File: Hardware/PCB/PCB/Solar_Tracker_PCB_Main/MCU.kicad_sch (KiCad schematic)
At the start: 20 parts, among them IC1 ESP32-S3-WROOM-1-N4R8, IC5 LM1117MPX-3.3_NOPB, J2 USB4940-00-A, J3 1729076, J4 1977223-1, J5 1977223-1

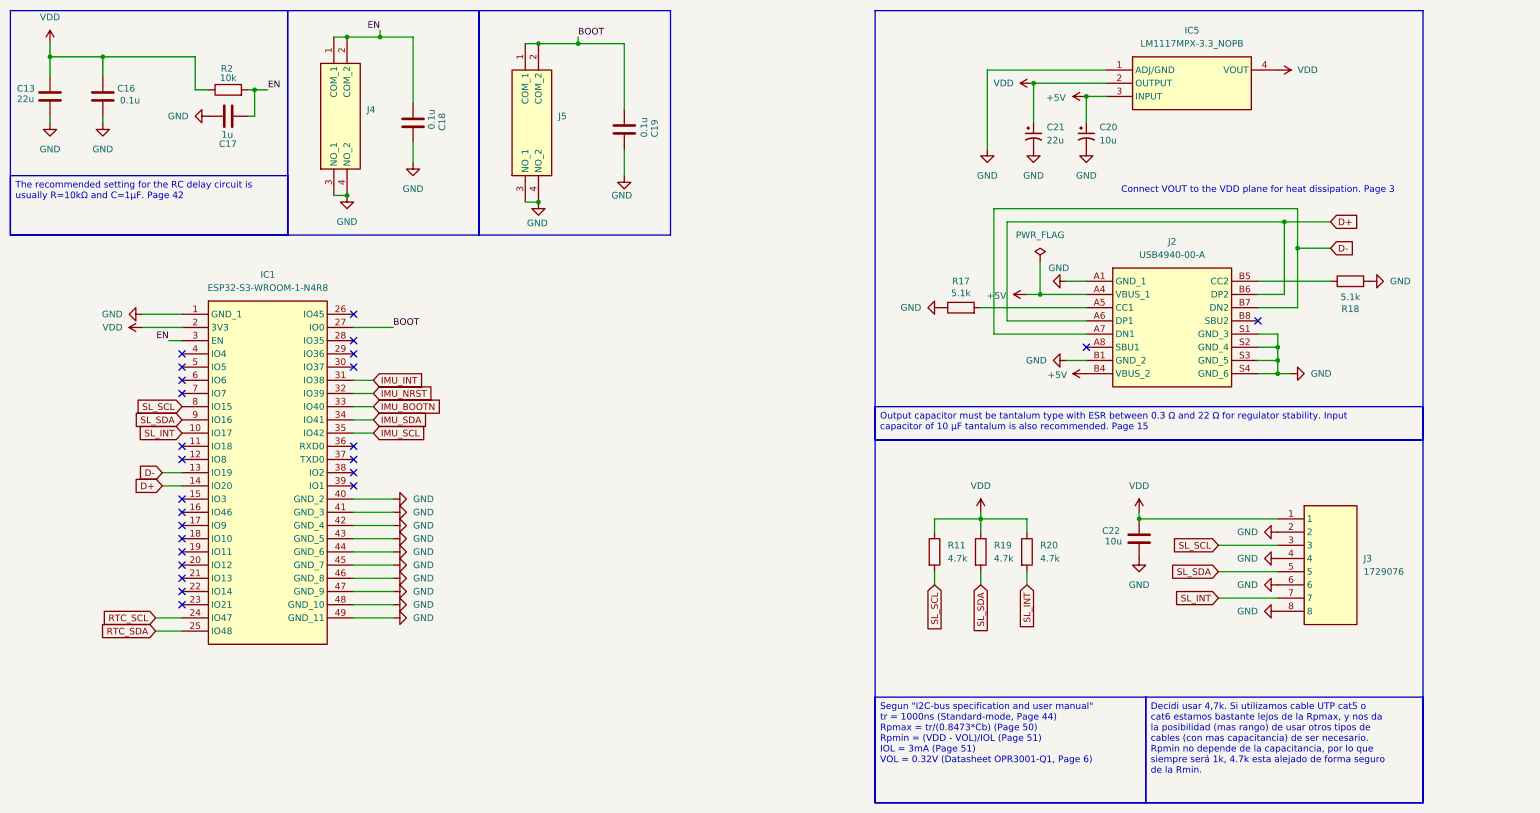
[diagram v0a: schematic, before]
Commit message: comienzo de distribucion pcb
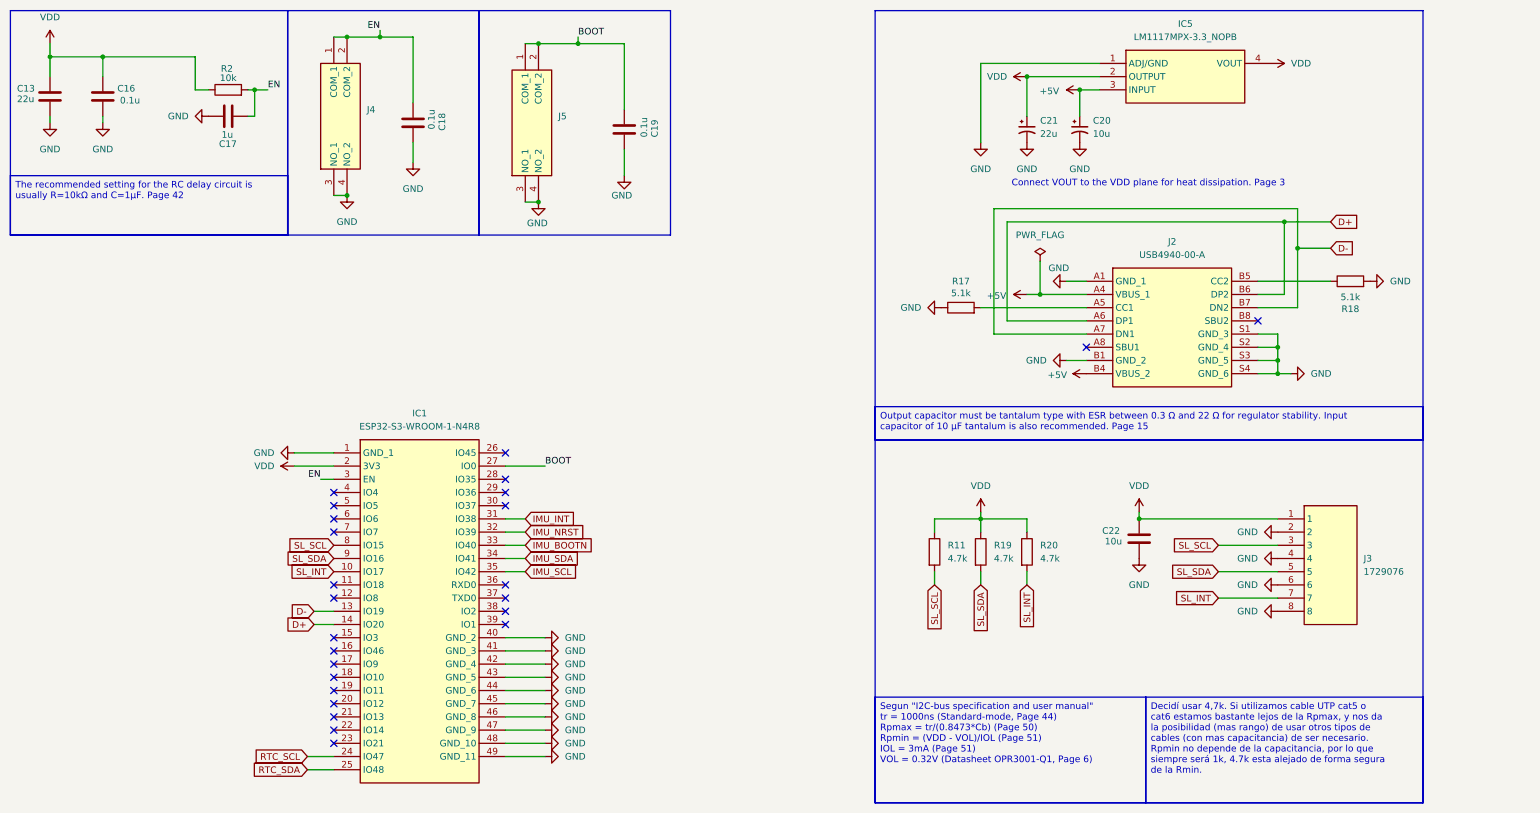
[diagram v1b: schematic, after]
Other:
- moved on the sheet: C20, C21, IC1, IC5

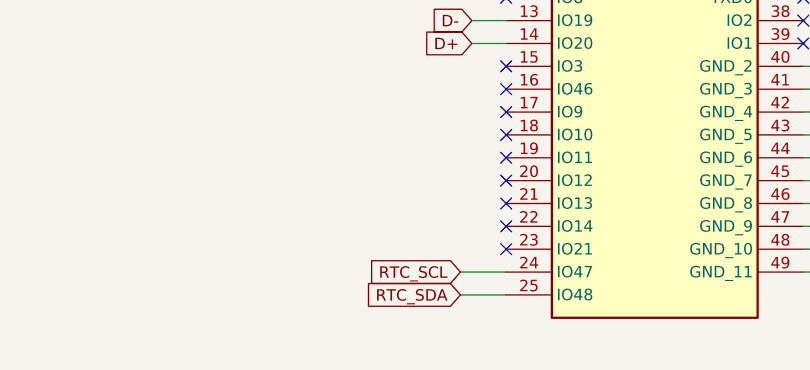
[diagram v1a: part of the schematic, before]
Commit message: Colocacion de los componentes en el PCB
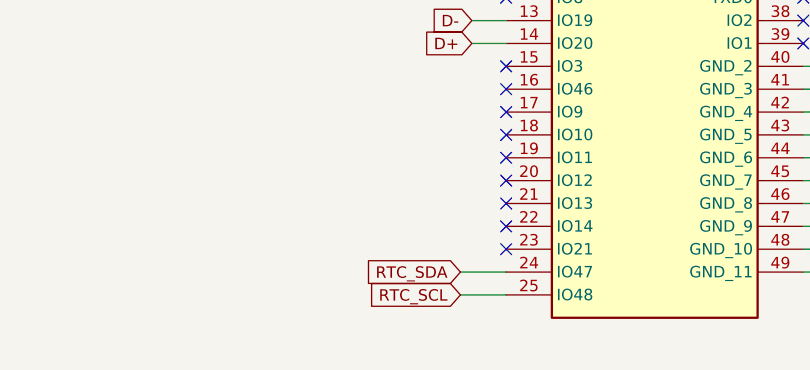
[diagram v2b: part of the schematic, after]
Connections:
- net RTC_SCL: now also IC1.25 (IO48); no longer IC1.24 (IO47)
- net RTC_SDA: now also IC1.24 (IO47); no longer IC1.25 (IO48)
